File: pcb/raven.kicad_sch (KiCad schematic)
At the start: 45 parts, among them J1 Conn_02x20_Odd_Even, J2 Conn_01x04_MountingPin, J3 Conn_01x02_Pin, J4 Conn_01x02_Pin, J5 Conn_01x04_MountingPin, J6 Conn_01x02_Pin, J7 Conn_01x02_Pin, J8 Conn_01x02_Pin, J9 Conn_01x02_Pin, U9 TPS548B28RWWR

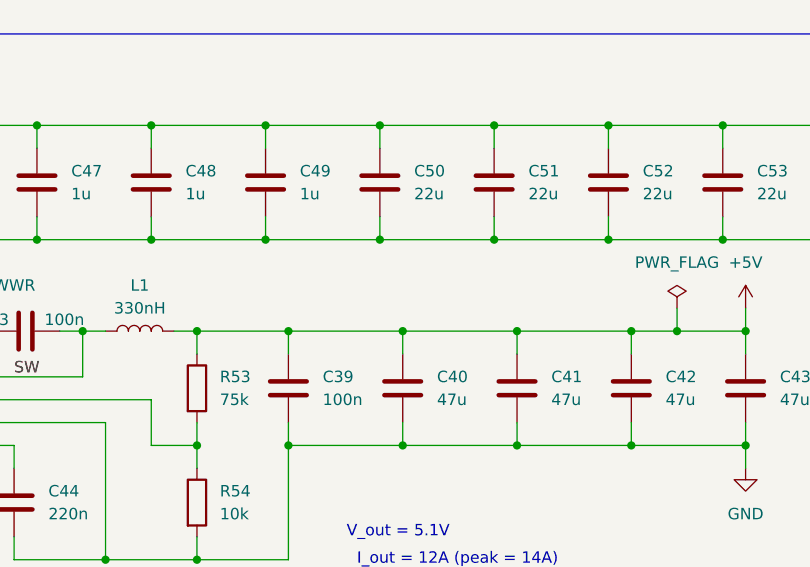
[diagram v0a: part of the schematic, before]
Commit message: Add new regulator info
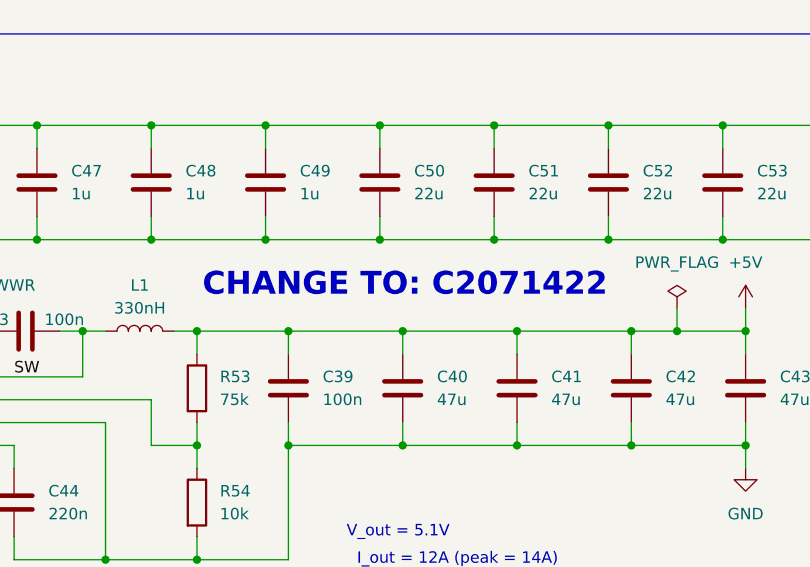
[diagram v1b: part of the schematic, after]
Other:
- note added: "CHANGE TO: C2071422"
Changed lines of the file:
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@@
+		)
+	)
+	(text "CHANGE TO: C2071422"
+		(exclude_from_sim no)
+		(at 203.454 119.38 0)
+		(effects
+			(font
+				(size 2.54 2.54)
+				(thickness 0.508)
+				(bold yes)
+			)
 		)
 	)

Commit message: Remove regulator
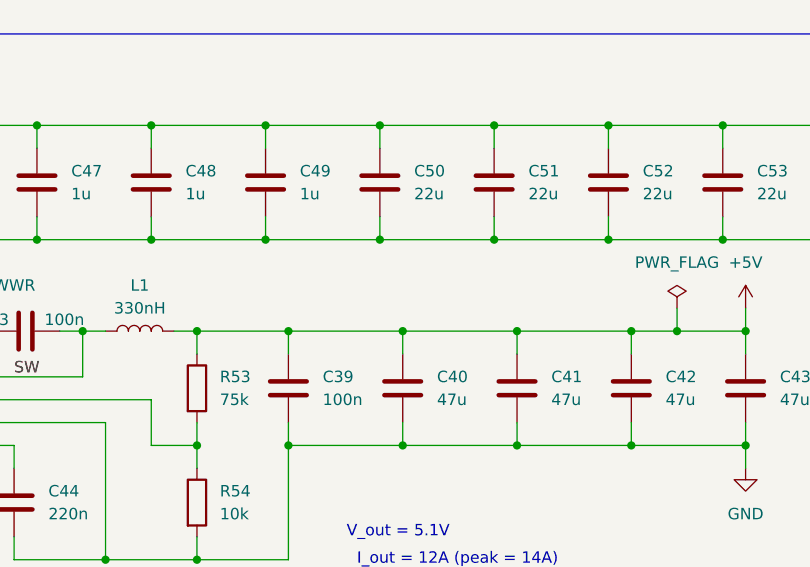
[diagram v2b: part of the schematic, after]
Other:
- note removed: "CHANGE TO: C2071422"
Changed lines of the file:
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@@
-		)
-	)
-	(text "CHANGE TO: C2071422"
-		(exclude_from_sim no)
-		(at 203.454 119.38 0)
-		(effects
-			(font
-				(size 2.54 2.54)
-				(thickness 0.508)
-				(bold yes)
-			)
 		)
 	)
